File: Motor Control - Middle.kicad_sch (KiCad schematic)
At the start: 9 parts, among them J3 BM09B-SRSS-TB, U11 TB9051FTG,EL

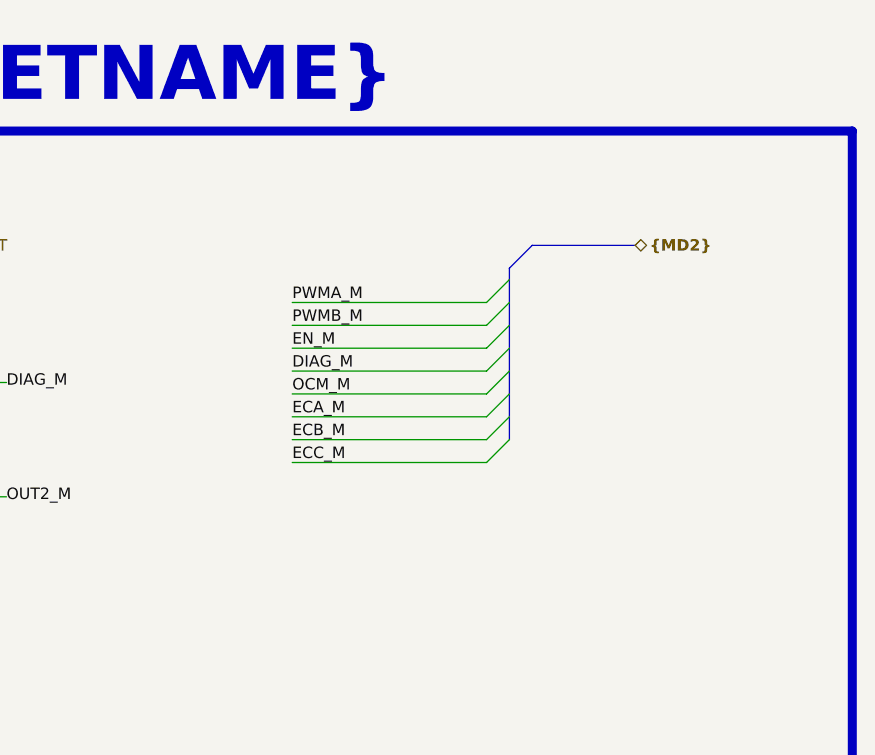
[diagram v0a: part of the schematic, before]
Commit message: Update Schematic
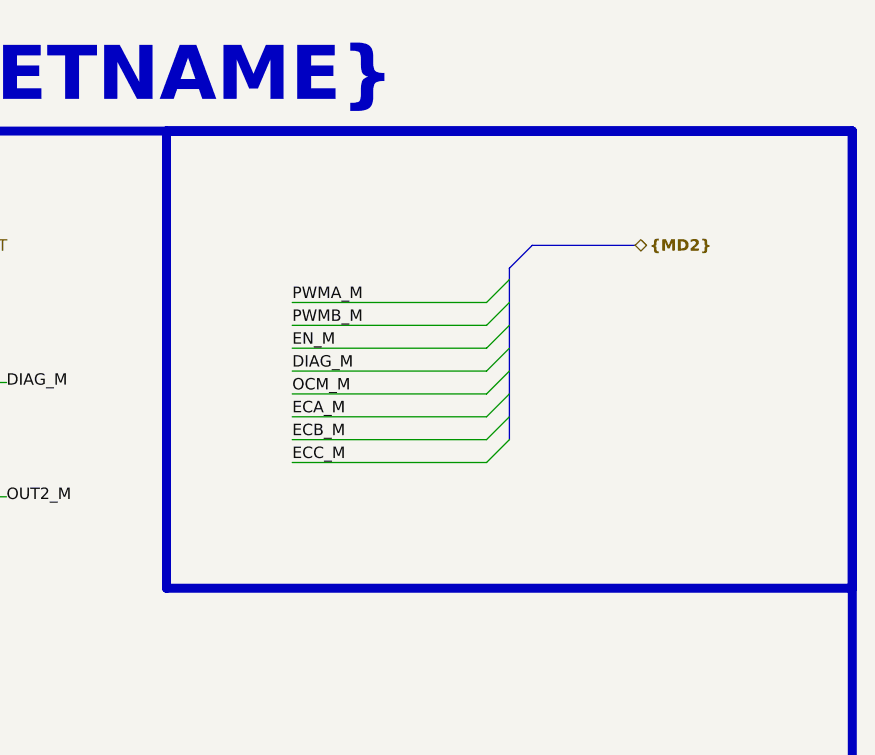
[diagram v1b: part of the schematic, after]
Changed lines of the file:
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@@
+		)
+	)
+	(rectangle
+		(start 177.8 25.4)
+		(end 254 76.2)
+		(stroke
+			(width 1)
+			(type default)
+			(color 200 0 0 1)
+		)
+		(fill
+			(type none)
 		)
 	)

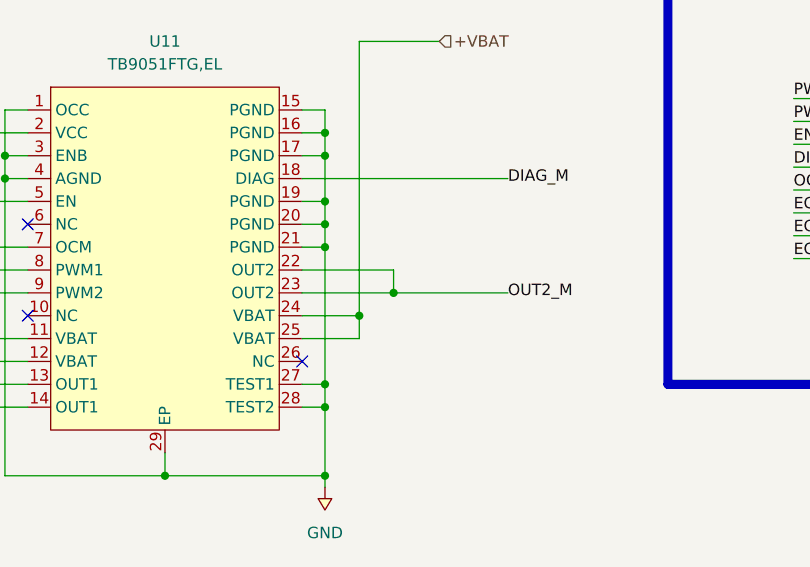
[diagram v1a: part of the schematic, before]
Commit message: Update Schematic
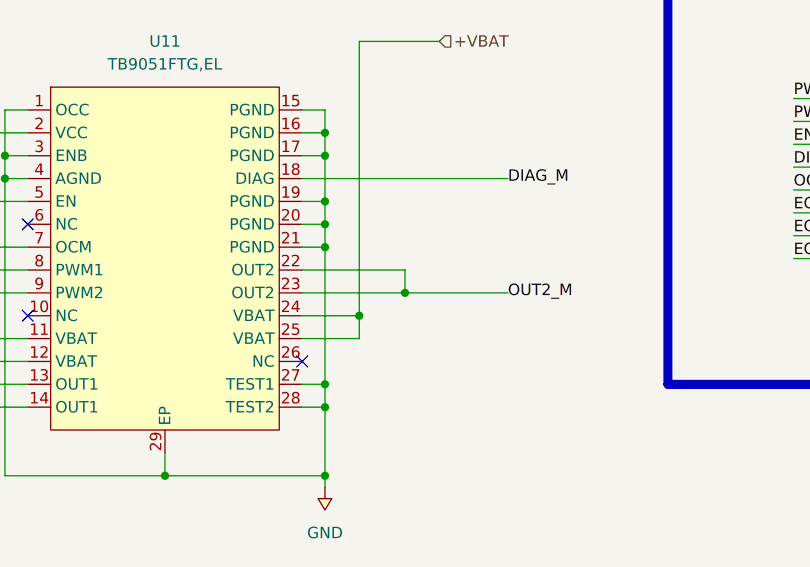
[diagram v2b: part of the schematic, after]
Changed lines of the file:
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@@
-	)
-	(junction
-		(at 147.32 66.04)
-		(diameter 0)
-		(color 0 0 0 0)
 	)
 	(junction
@@
 	(junction
 		(at 66.04 129.54)
+		(diameter 0)
+		(color 0 0 0 0)
+	)
+	(junction
+		(at 148.59 66.04)
 		(diameter 0)
 		(color 0 0 0 0)
@@
 	(wire
 		(pts
-			(xy 137.16 66.04) (xy 147.32 66.04)
+			(xy 137.16 66.04) (xy 148.59 66.04)
 		)
 		(stroke
@@
 	(wire
 		(pts
-			(xy 147.32 63.5) (xy 147.32 66.04)
+			(xy 148.59 63.5) (xy 148.59 66.04)
 		)
 		(stroke
@@
 	(wire
 		(pts
-			(xy 147.32 66.04) (xy 160.02 66.04)
-		)
-		(stroke
-			(width 0)
-			(type default)
-		)
-	)
-	(wire
-		(pts
 			(xy 88.9 127) (xy 88.9 129.54)
 		)
@@
 	(wire
 		(pts
+			(xy 148.59 66.04) (xy 160.02 66.04)
+		)
+		(stroke
+			(width 0)
+			(type default)
+		)
+	)
+	(wire
+		(pts
 			(xy 231.14 119.38) (xy 234.95 119.38)
 		)
@@
 	(wire
 		(pts
-			(xy 137.16 63.5) (xy 147.32 63.5)
-		)
-		(stroke
+			(xy 137.16 63.5) (xy 148.59 63.5)
+		)
+		(stroke

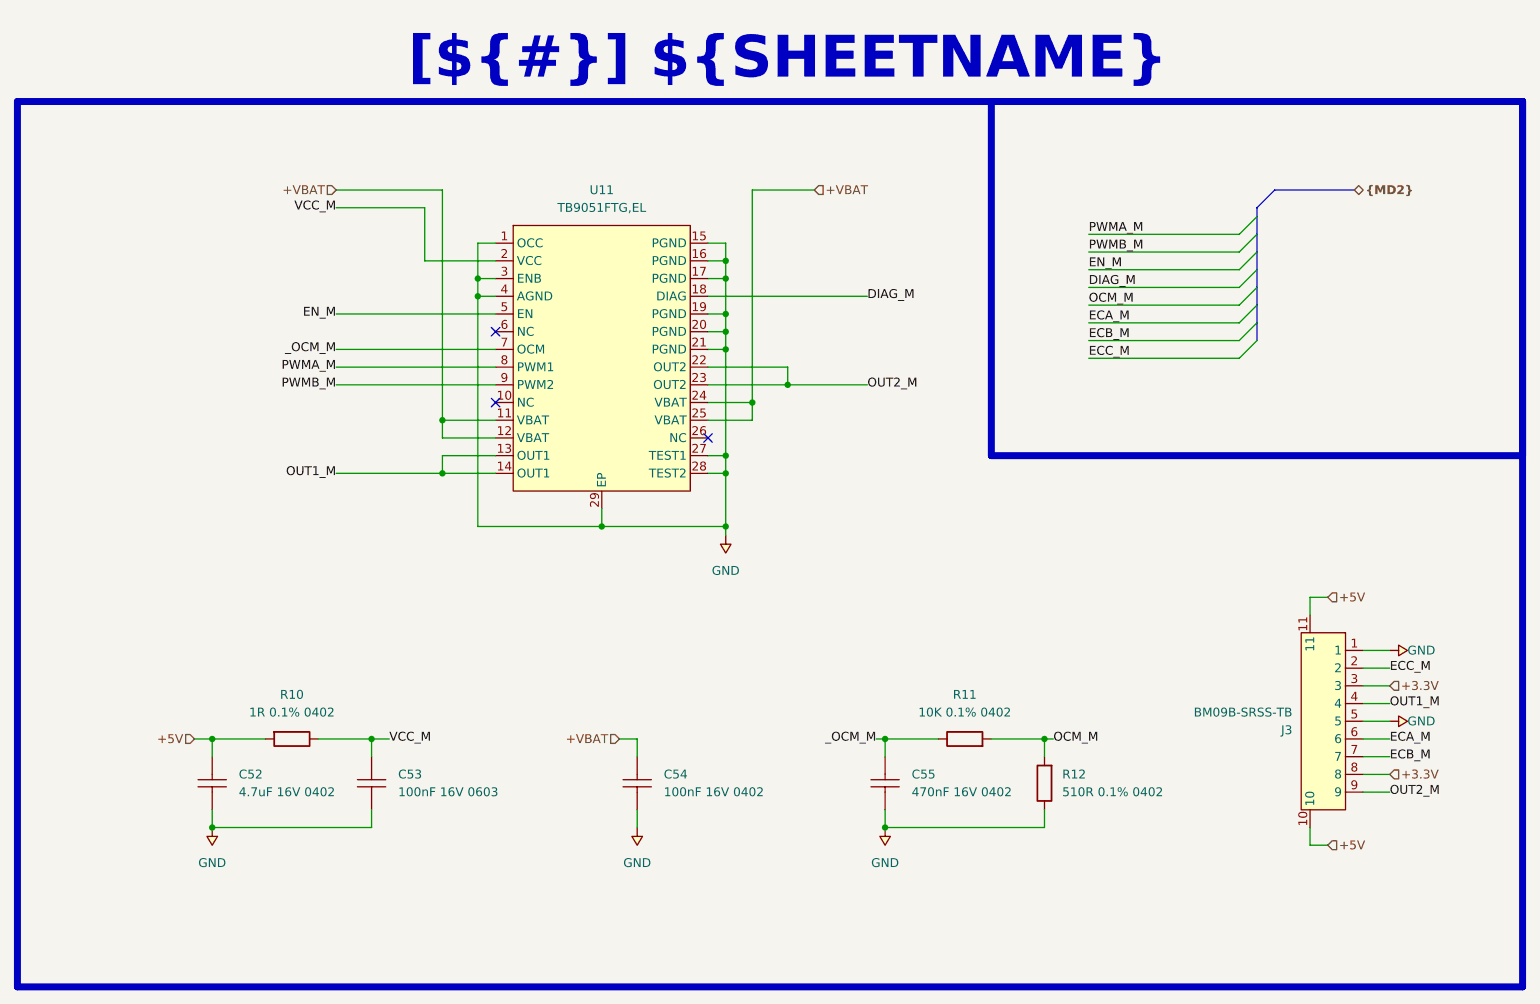
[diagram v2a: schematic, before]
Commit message: Update Schematic
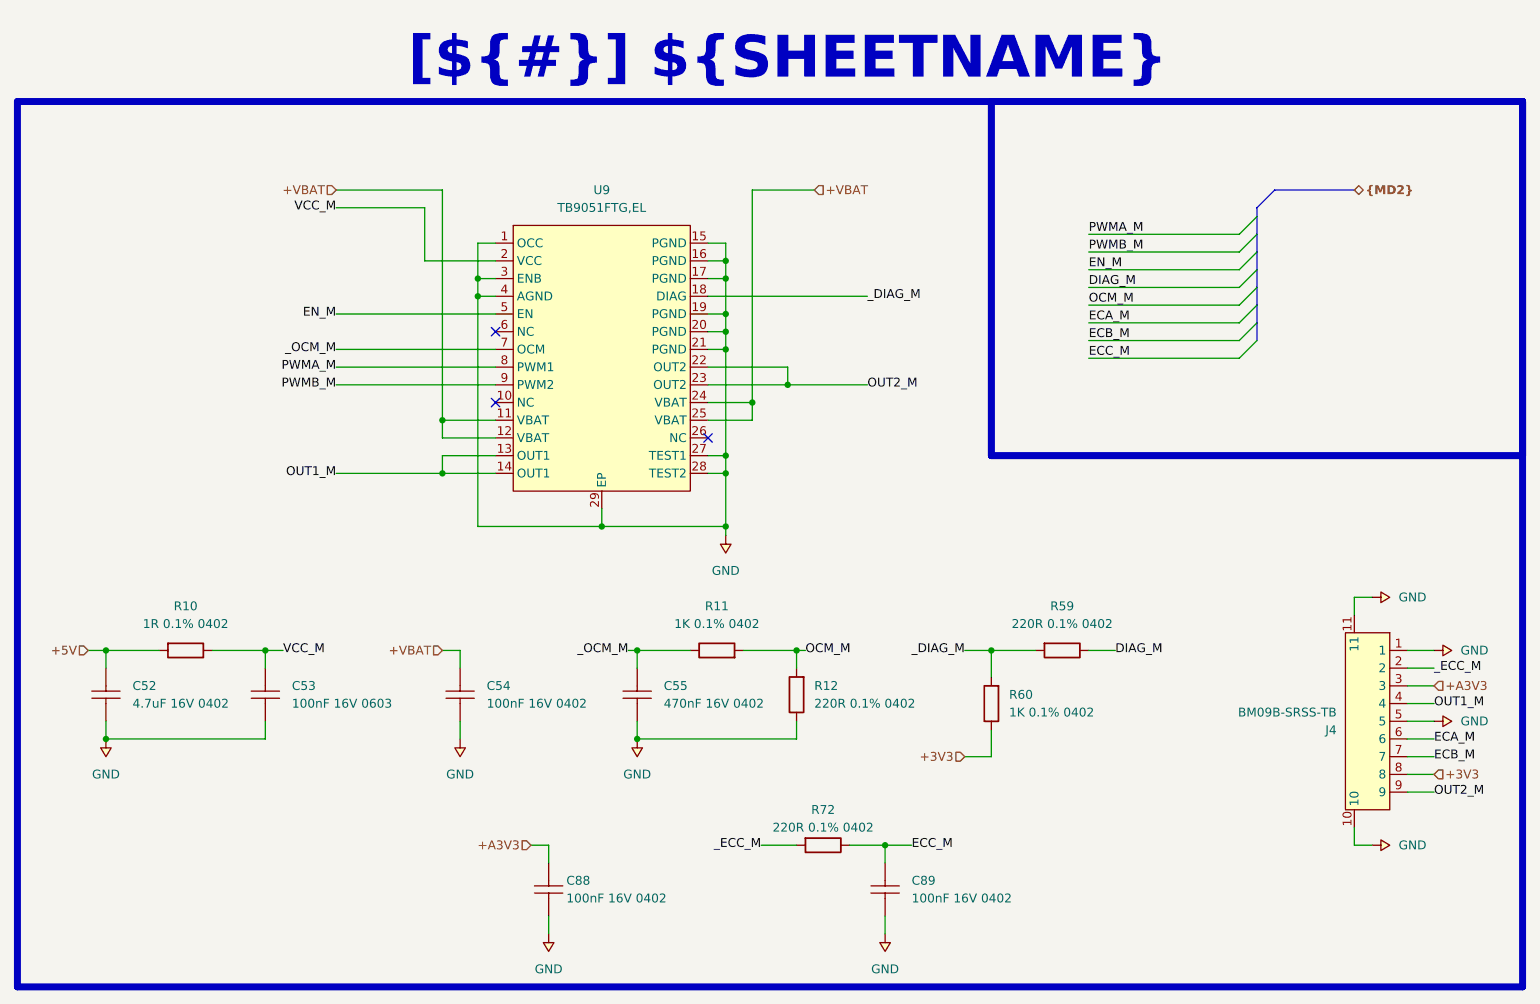
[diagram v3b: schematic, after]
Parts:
- removed J3: BM09B-SRSS-TB, Duc:CONN-SMD_9P-P1.00_BM09B-SRSS-TB, symbol Duc-Connectors:BM09B-SRSS-TB
- added C88, C89: 100nF 16V 0402, Duc_Library:C0402, symbol Duc-Capacitors:CAP CER 0402
- added J4: BM09B-SRSS-TB, Duc:CONN-SMD_9P-P1.00_BM09B-SRSS-TB, symbol Duc-Connectors:BM09B-SRSS-TB
- added R59, R72: 220R 0.1% 0402, Duc_Library:R0402, symbol Duc-Resistors:RES SMD 0402
- added R60: 1K 0.1% 0402, Duc_Library:R0402, symbol Duc-Resistors:RES SMD 0402
- R11: value 10K 0.1% 0402 -> 1K 0.1% 0402
- R12: value 510R 0.1% 0402 -> 220R 0.1% 0402
- renumbered U11 to U9
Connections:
- net DIAG_M: now also R59.2; no longer U9.18 (DIAG)
- net ECA_M: now also J4.6
- net ECB_M: now also J4.7
- net ECC_M: now also C89.2, R72.2
- net GND: now also C88.1, C89.1, J4.1, J4.10, J4.11, J4.5
- net OUT1_M: now also J4.4
- net OUT2_M: now also J4.9
- new net +3V3: J4.8, R60.2
- new net +A3V3: C88.2, J4.3
- new net _DIAG_M: R59.1, R60.1, U9.18 (DIAG)
- new net _ECC_M: J4.2, R72.1
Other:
- moved on the sheet: C52, C53, C54, C55, R10, R11, R12
